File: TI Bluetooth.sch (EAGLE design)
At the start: 43 parts, among them J1 DEBUG Connector, J2 USB Type C Connector, J3 Expansion Header, U1 TPS62160, U2 CC2642R, Y1 32.768kHz, Y2 48MHz

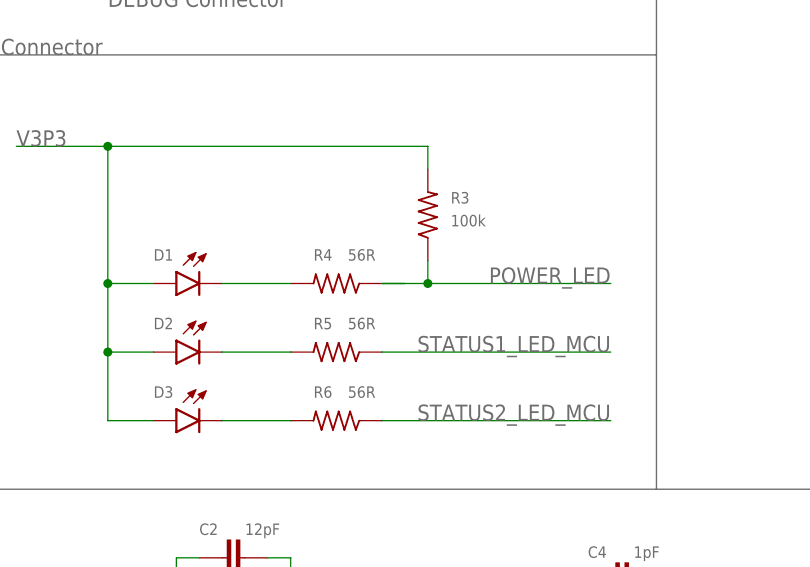
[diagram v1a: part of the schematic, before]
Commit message: Much of routing finished
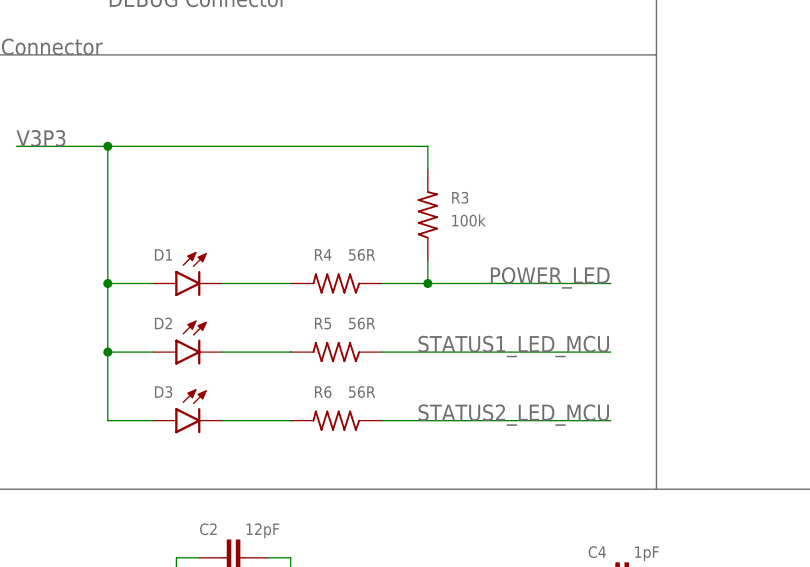
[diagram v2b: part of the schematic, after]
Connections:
- removed net N$24: ANT1.FEED, C6.2
- net GND: now also ANT1.FEED, C6.2
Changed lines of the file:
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@@
-</segment>
-</net>
-<net name="N$24" class="0">
-<segment>
-<pinref part="C6" gate="G$1" pin="2"/>
-<pinref part="ANT1" gate="ANT_2.4GHZ" pin="FEED"/>
-<wire x1="-205.74" y1="965.2" x2="-215.9" y2="965.2" width="0.1524" layer="91"/>
 </segment>
 </net>
@@
 </segment>
 <segment>
-<pinref part="R4" gate="G$1" pin="1"/>
-<wire x1="-274.32" y1="1018.54" x2="-271.78" y2="1018.54" width="0.1524" layer="91"/>
 <wire x1="-248.92" y1="1018.54" x2="-269.24" y2="1018.54" width="0.1524" layer="91"/>
 <label x="-248.92" y="1018.54" size="1.778" layer="95" align="bottom-right"/>
 <pinref part="R3" gate="G$1" pin="1"/>
-<wire x1="-269.24" y1="1018.54" x2="-274.32" y2="1018.54" width="0.1524" layer="91"/>
 <wire x1="-269.24" y1="1021.08" x2="-269.24" y2="1018.54" width="0.1524" layer="91"/>
+<pinref part="R4" gate="G$1" pin="1"/>
+<wire x1="-274.32" y1="1018.54" x2="-269.24" y2="1018.54" width="0.1524" layer="91"/>
 <junction x="-269.24" y="1018.54"/>
 </segment>
@@
 <pinref part="SUPPLY7" gate="GND" pin="GND"/>
 </segment>
-</net>
+<segment>
+<pinref part="C6" gate="G$1" pin="2"/>
+<pinref part="ANT1" gate="ANT_2.4GHZ" pin="FEED"/>
+<wire x1="-205.74" y1="965.2" x2="-215.9" y2="965.2" width="0.1524" layer="91"/>
+</segment>
+</net>
